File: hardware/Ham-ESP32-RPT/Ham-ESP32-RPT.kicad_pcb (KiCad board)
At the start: 2 copper layers, 115 x 100 mm, 26 parts, among them J1 5V SUPPLY, J2 12V SUPPLY, J3 RX RADIO, J4 TX RADIO, J5 AUX BTN LED, J6 SPEAKER, Q1 MMBT2222A, SW2 TEST, U1 ESP32-S3-DevKitC-V2, U2 PmodI2S2, U3 INA219AxD

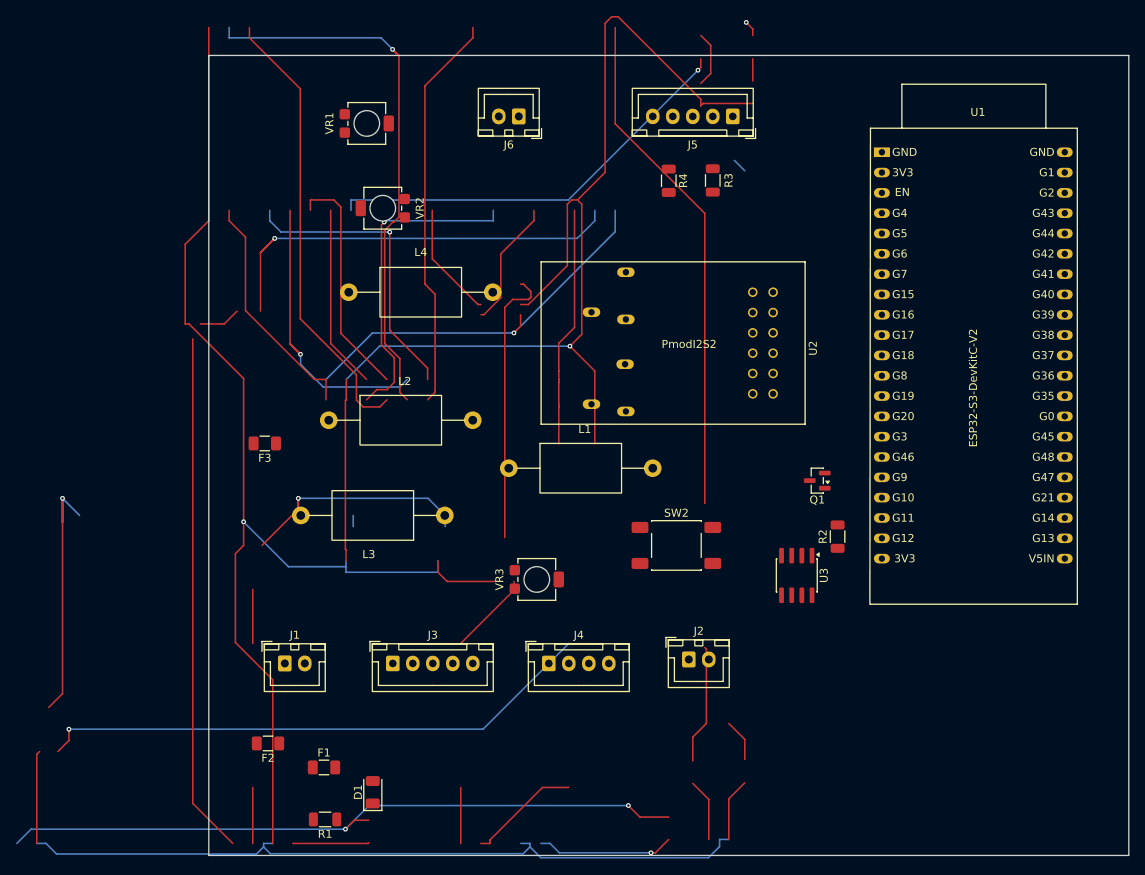
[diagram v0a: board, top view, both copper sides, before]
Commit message: PCB Update
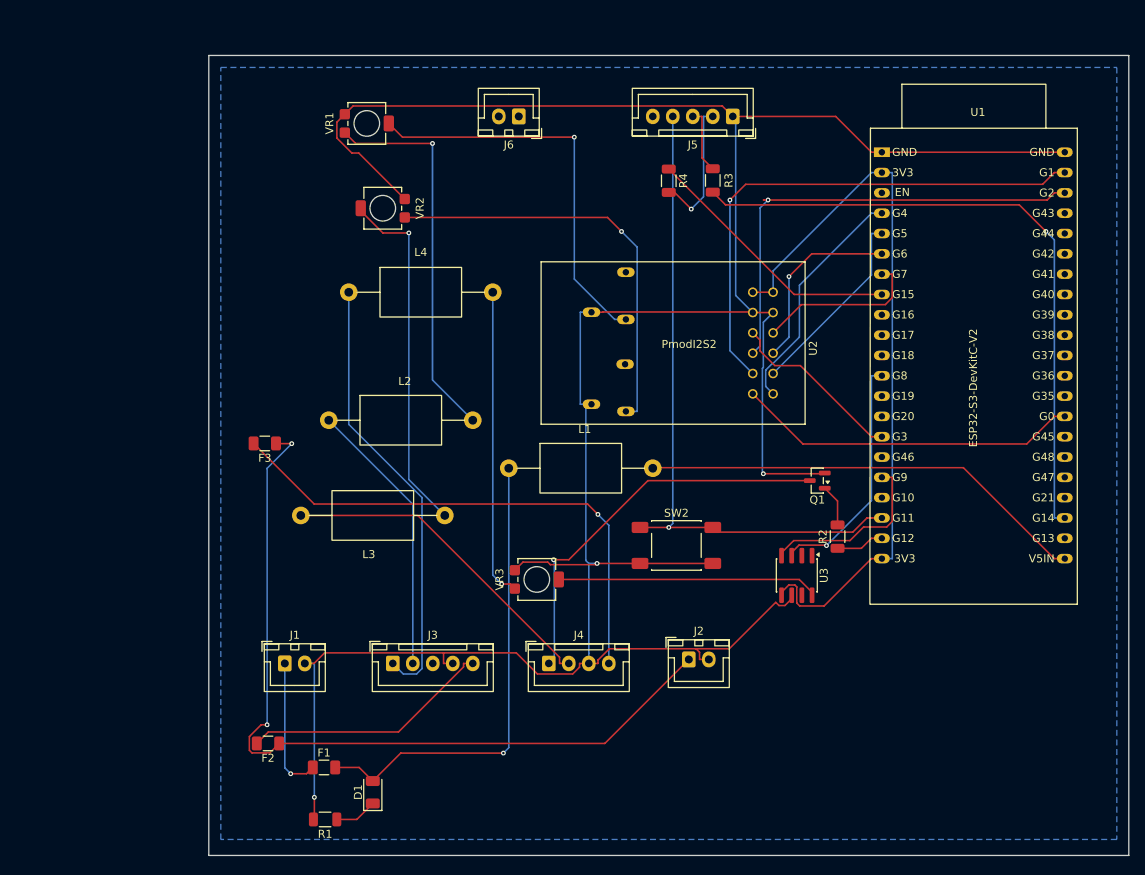
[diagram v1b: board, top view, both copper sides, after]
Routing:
- net GND: track 481.5 -> 351.4 mm, vias 2 -> 3
- net Net-(J5-Pin_4): track 0.00 -> 82.8 mm, vias 0 -> 1
- net Net-(U1-G14): track 0.00 -> 81.2 mm, vias 0 -> 1
- net Net-(U1-G1): track 0.00 -> 66.7 mm, vias 0 -> 1
- net Net-(U1-G2): track 0.00 -> 58.5 mm, vias 0 -> 1
- net Net-(J4-Pin_4): track 9.54 -> 65.9 mm, vias 0 -> 1
- net Net-(U1-G12): track 62.1 -> 6.06 mm, vias 1 -> 0
- net unconnected-(J5-Pin_5-Pad5): track 53.0 -> 0.00 mm, vias 1 -> 0
- net Net-(U2-A_OUT_L): track 0.00 -> 52.5 mm, vias 0 -> 1
- net Net-(U2-A_IN_L): track 0.00 -> 50.2 mm, vias 0 -> 1
- net Net-(J2-Pin_1): track 152.6 -> 103.0 mm
- net Net-(L2-Pad2): track 0.00 -> 48.2 mm, vias 0 -> 1
- net unconnected-(J3-Pin_3-Pad3): track 43.4 -> 0.00 mm, vias 1 -> 0
- net Net-(U1-G0): track 0.00 -> 43.0 mm
- net Net-(L3-Pad1): track 6.75 -> 44.7 mm, vias 0 -> 1
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- added copper zone on B.Cu, net GND
